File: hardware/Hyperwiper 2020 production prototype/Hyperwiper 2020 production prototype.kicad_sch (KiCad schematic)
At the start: 19 parts, among them K1 Main Power relay, K2 Wiper control relay, Q1 PN2222A, SW1 ON-OFF, U1 Teensy4.0, U3 L7805

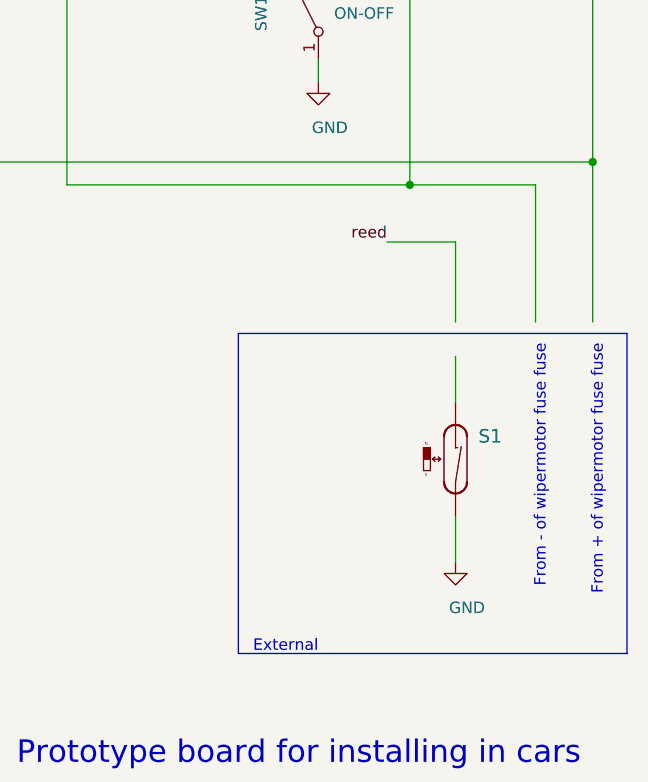
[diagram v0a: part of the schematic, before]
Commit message: Updated Schematic and board.
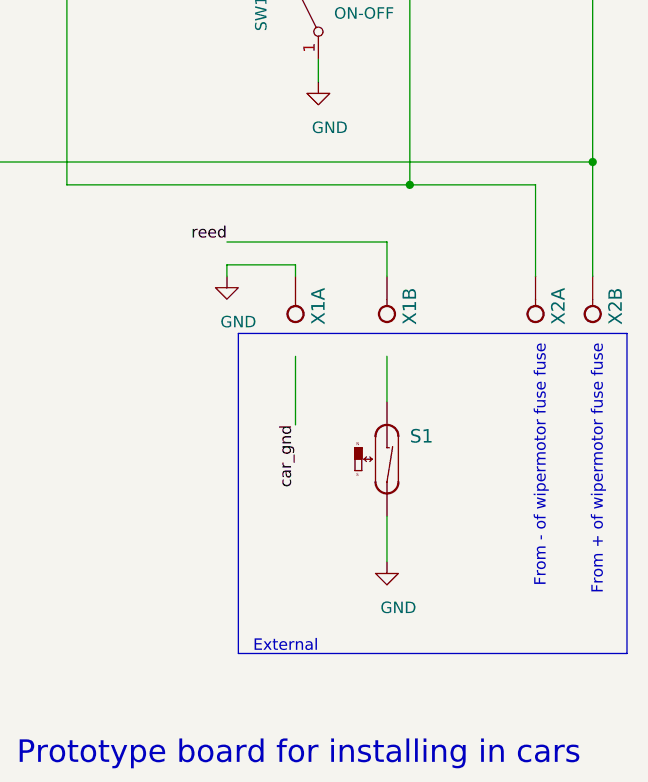
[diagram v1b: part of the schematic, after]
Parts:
- added X1, X2: W237-3E-bGeigieNanoKit_V1.1r5a-eagle-import, DWP 2020:W237-3E, symbol import_from_eagle-rescue:W237-3E-bGeigieNanoKit_V1.1r5a-eagle-import
- RV1: footprint Potentiometer_THT:Potentiometer_Alps_RK09K_Single_Horizontal -> Potentiometer_THT:Potentiometer_Piher_PT-10-V05_Vertical
- U3: footprint Package_TO_SOT_THT:TO-220-3_Vertical -> Package_TO_SOT_THT:TO-220-3_Horizontal_TabUp
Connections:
- net GND: now also X1.1 (KL)
- net reed: now also X1.2 (KL)
- net at K1.1, K2.3: now also X2.1 (KL)
- net at K1.4, K1.5, K2.1: now also X2.2 (KL)
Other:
- moved on the sheet: S1
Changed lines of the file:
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@@
+    (stroke (width 0) (type solid) (color 0 0 0 0))
+  )
+  (wire (pts (xy 234.95 114.3) (xy 252.73 114.3))
+    (stroke (width 0) (type solid) (color 0 0 0 0))
+  )
+  (wire (pts (xy 234.95 116.84) (xy 242.57 116.84))
+    (stroke (width 0) (type solid) (color 0 0 0 0))
+  )
+  (wire (pts (xy 234.95 118.11) (xy 234.95 116.84))
     (stroke (width 0) (type solid) (color 0 0 0 0))
   )
@@
     (stroke (width 0) (type solid) (color 0 0 0 0))
   )
+  (wire (pts (xy 242.57 116.84) (xy 242.57 118.11))
+    (stroke (width 0) (type solid) (color 0 0 0 0))
+  )
+  (wire (pts (xy 242.57 127) (xy 242.57 134.62))
+    (stroke (width 0) (type solid) (color 0 0 0 0))
+  )
   (wire (pts (xy 245.11 52.07) (xy 252.73 52.07))
     (stroke (width 0) (type solid) (color 0 0 0 0))
@@
     (stroke (width 0) (type solid) (color 0 0 0 0))
   )
-  (wire (pts (xy 252.73 114.3) (xy 260.35 114.3))
+  (wire (pts (xy 252.73 114.3) (xy 252.73 118.11))
+    (stroke (width 0) (type solid) (color 0 0 0 0))
+  )
+  (wire (pts (xy 252.73 127) (xy 252.73 132.08))
+    (stroke (width 0) (type solid) (color 0 0 0 0))
+  )
+  (wire (pts (xy 252.73 144.78) (xy 252.73 149.86))
     (stroke (width 0) (type solid) (color 0 0 0 0))
   )
@@
     (stroke (width 0) (type solid) (color 0 0 0 0))
   )
-  (wire (pts (xy 260.35 123.19) (xy 260.35 114.3))
-    (stroke (width 0) (type solid) (color 0 0 0 0))
-  )
-  (wire (pts (xy 260.35 127) (xy 260.35 132.08))
-    (stroke (width 0) (type solid) (color 0 0 0 0))
-  )
-  (wire (pts (xy 260.35 144.78) (xy 260.35 149.86))
-    (stroke (width 0) (type solid) (color 0 0 0 0))
-  )
-  (wire (pts (xy 269.24 107.95) (xy 269.24 123.19))
+  (wire (pts (xy 269.24 107.95) (xy 269.24 118.11))
     (stroke (width 0) (type solid) (color 0 0 0 0))
   )
@@
     (stroke (width 0) (type solid) (color 0 0 0 0))
   )
-  (wire (pts (xy 275.59 105.41) (xy 275.59 123.19))
+  (wire (pts (xy 275.59 105.41) (xy 275.59 118.11))
     (stroke (width 0) (type solid) (color 0 0 0 0))
   )
@@
     (effects (font (size 1.27 1.27)) (justify right bottom))
   )
+  (label "reed" (at 234.95 114.3 180)
+    (effects (font (size 1.27 1.27)) (justify right bottom))
+  )
+  (label "car_gnd" (at 242.57 134.62 270)
+    (effects (font (size 1.27 1.27)) (justify right bottom))
+  )
   (label "5V" (at 248.92 20.32 180)
     (effects (font (size 1.27 1.27)) (justify right bottom))
   )
-  (label "reed" (at 252.73 114.3 180)
-    (effects (font (size 1.27 1.27)) (justify right bottom))
-  )
   (symbol (lib_id "power:GND") (at 118.11 86.36 0) (unit 1)
     (in_bom yes) (on_board yes)
-    (property "Reference" "#PWR?" (id 0) (at 118.11 92.71 0)
+    (property "Reference" "#PWR0109" (id 0) (at 118.11 92.71 0)
       (effects (font (size 1.27 1.27)) hide)
     )
@@
     )
   )
+  (symbol (lib_id "power:GND") (at 234.95 118.11 0) (unit 1)
+    (in_bom yes) (on_board yes)
+    (property "Reference" "#PWR0110" (id 0) (at 234.95 124.46 0)
+      (effects (font (size 1.27 1.27)) hide)
+    )
+    (property "Value" "GND" (id 1) (at 236.22 123.19 0))
+    (property "Footprint" "" (id 2) (at 234.95 118.11 0)
+      (effects (font (size 1.27 1.27)) hide)
+    )
+    (property "Datasheet" "" (id 3) (at 234.95 118.11 0)
+      (effects (font (size 1.27 1.27)) hide)
+    )
+  )
   (symbol (lib_id "power:GND") (at 241.3 40.64 0) (unit 1)
     (in_bom yes) (on_board yes)
@@
     )
   )
-  (symbol (lib_id "power:GND") (at 260.35 149.86 0) (unit 1)
-    (in_bom yes) (on_board yes)
-    (property "Reference" "#PWR0104" (id 0) (at 260.35 156.21 0)
-      (effects (font (size 1.27 1.27)) hide)
-    )
-    (property "Value" "GND" (id 1) (at 261.62 154.94 0))
-    (property "Footprint" "" (id 2) (at 260.35 149.86 0)
-      (effects (font (size 1.27 1.27)) hide)
-    )
-    (property "Datasheet" "" (id 3) (at 260.35 149.86 0)
+  (symbol (lib_id "power:GND") (at 252.73 149.86 0) (unit 1)
+    (in_bom yes) (on_board yes)
+    (property "Reference" "#PWR0104" (id 0) (at 252.73 156.21 0)
+      (effects (font (size 1.27 1.27)) hide)
+    )
+    (property "Value" "GND" (id 1) (at 254 154.94 0))
+    (property "Footprint" "" (id 2) (at 252.73 149.86 0)
+      (effects (font (size 1.27 1.27)) hide)
+    )
+    (property "Datasheet" "" (id 3) (at 252.73 149.86 0)
+      (effects (font (size 1.27 1.27)) hide)
+    )
+  )
+  (symbol (lib_id "import_from_eagle-rescue:W237-3E-bGeigieNanoKit_V1.1r5a-eagle-import") (at 242.57 123.19 90) (unit 1)
+    (in_bom yes) (on_board yes)
+    (property "Reference" "X1" (id 0) (at 245.11 119.38 0)
+      (effects (font (size 1.4986 1.4986)) (justify right))
+    )
+    (property "Value" "W237-3E-bGeigieNanoKit_V1.1r5a-eagle-import" (id 1) (at 245.11 121.92 90)
+      (effects (font (size 1.499 1.499)) (justify right) hide)
+    )
+    (property "Footprint" "DWP 2020:W237-3E" (id 2) (at 242.57 123.19 0)
+      (effects (font (size 1.27 1.27)) hide)
+    )
+    (property "Datasheet" "" (id 3) (at 242.57 123.19 0)
+      (effects (font (size 1.27 1.27)) hide)
+    )
+  )
+  (symbol (lib_id "import_from_eagle-rescue:W237-3E-bGeigieNanoKit_V1.1r5a-eagle-import") (at 252.73 123.19 90) (unit 2)
+    (in_bom yes) (on_board yes)
+    (property "Reference" "X1" (id 0) (at 255.27 119.38 0)
+      (effects (font (size 1.4986 1.4986)) (justify right))
+    )
+    (property "Value" "W237-3E-bGeigieNanoKit_V1.1r5a-eagle-import" (id 1) (at 255.27 121.92 90)
+      (effects (font (size 1.499 1.499)) (justify right) hide)
+    )
+    (property "Footprint" "DWP 2020:W237-3E" (id 2) (at 252.73 123.19 0)
+      (effects (font (size 1.27 1.27)) hide)
+    )
+    (property "Datasheet" "" (id 3) (at 252.73 123.19 0)
+      (effects (font (size 1.27 1.27)) hide)
+    )
+  )
+  (symbol (lib_id "import_from_eagle-rescue:W237-3E-bGeigieNanoKit_V1.1r5a-eagle-import") (at 269.24 123.19 90) (unit 1)
+    (in_bom yes) (on_board yes)
+    (property "Reference" "X2" (id 0) (at 271.78 119.38 0)
+      (effects (font (size 1.4986 1.4986)) (justify right))
+    )
+    (property "Value" "W237-3E-bGeigieNanoKit_V1.1r5a-eagle-import" (id 1) (at 271.78 121.92 90)
+      (effects (font (size 1.499 1.499)) (justify right) hide)
+    )
+    (property "Footprint" "DWP 2020:W237-3E" (id 2) (at 269.24 123.19 0)
+      (effects (font (size 1.27 1.27)) hide)
+    )
+    (property "Datasheet" "" (id 3) (at 269.24 123.19 0)
+      (effects (font (size 1.27 1.27)) hide)
+    )
+  )
+  (symbol (lib_id "import_from_eagle-rescue:W237-3E-bGeigieNanoKit_V1.1r5a-eagle-import") (at 275.59 123.19 90) (unit 2)
+    (in_bom yes) (on_board yes)
+    (property "Reference" "X2" (id 0) (at 278.13 119.38 0)
+      (effects (font (size 1.4986 1.4986)) (justify right))
+    )
+    (property "Value" "W237-3E-bGeigieNanoKit_V1.1r5a-eagle-import" (id 1) (at 278.13 121.92 90)
+      (effects (font (size 1.499 1.499)) (justify right) hide)
+    )
+    (property "Footprint" "DWP 2020:W237-3E" (id 2) (at 275.59 123.19 0)
+      (effects (font (size 1.27 1.27)) hide)
+    )
+    (property "Datasheet" "" (id 3) (at 275.59 123.19 0)
       (effects (font (size 1.27 1.27)) hide)
     )
@@
       (effects (font (size 1.27 1.27)) (justify right))
     )
-    (property "Footprint" "Potentiometer_THT:Potentiometer_Alps_RK09K_Single_Horizontal" (id 2) (at 161.29 160.02 0)
+    (property "Footprint" "Potentiometer_THT:Potentiometer_Piher_PT-10-V05_Vertical" (id 2) (at 161.29 160.02 0)
       (effects (font (size 1.27 1.27)) hide)
     )
@@
     )
   )
-  (symbol (lib_id "import_from_eagle-rescue:REED-SWITCH-CT10-A2-bGeigieNanoKit_V1.1r5a-eagle-import") (at 260.35 139.7 0) (unit 1)
-    (in_bom yes) (on_board yes)
-    (property "Reference" "S1" (id 0) (at 262.89 135.89 0)
+  (symbol (lib_id "import_from_eagle-rescue:REED-SWITCH-CT10-A2-bGeigieNanoKit_V1.1r5a-eagle-import") (at 252.73 139.7 0) (unit 1)
+    (in_bom yes) (on_board yes)
+    (property "Reference" "S1" (id 0) (at 255.27 135.89 0)
       (effects (font (size 1.4986 1.4986)) (justify left))
     )
-    (property "Value" "REED-SWITCH-CT10-A2-bGeigieNanoKit_V1.1r5a-eagle-import" (id 1) (at 262.89 139.7 0)
+    (property "Value" "REED-SWITCH-CT10-A2-bGeigieNanoKit_V1.1r5a-eagle-import" (id 1) (at 255.27 139.7 0)
       (effects (font (size 1.499 1.499)) (justify left) hide)
     )
-    (property "Footprint" "" (id 2) (at 260.35 139.7 0)
-      (effects (font (size 1.27 1.27)) hide)
-    )
-    (property "Datasheet" "" (id 3) (at 260.35 139.7 0)
+    (property "Footprint" "" (id 2) (at 252.73 139.7 0)
+      (effects (font (size 1.27 1.27)) hide)
+    )
+    (property "Datasheet" "" (id 3) (at 252.73 139.7 0)
       (effects (font (size 1.27 1.27)) hide)
     )
@@
     (property "Reference" "U3" (id 0) (at 241.3 21.59 0))
     (property "Value" "L7805" (id 1) (at 241.3 24.13 0))
-    (property "Footprint" "Package_TO_SOT_THT:TO-220-3_Vertical" (id 2) (at 241.935 33.02 0)
+    (property "Footprint" "Package_TO_SOT_THT:TO-220-3_Horizontal_TabUp" (id 2) (at 241.935 33.02 0)
       (effects (font (size 1.27 1.27) italic) (justify left) hide)
     )
@@
     )
     (path "/9b49453a-7d8c-46f7-ac72-5b7ca2259e26"
-      (reference "#PWR?") (unit 1)
+      (reference "#PWR0109") (unit 1)
+    )
+    (path "/8e8791e7-f5c8-46ac-8494-bdb46b4d3074"
+      (reference "#PWR0110") (unit 1)
     )
     (path "/3e7c7f71-990b-4b23-8faa-21bc92ed5e62"
@@
       (reference "U3") (unit 1)
     )
-  )
+    (path "/a84228e8-43cd-4089-b680-2e81d592d20a"
+      (reference "X1") (unit 1)
+    )
+    (path "/20235294-3224-4d0b-9ea7-1bc2750028c9"
+      (reference "X1") (unit 2)
+    )
+    (path "/7b8a6e5c-ae62-44de-ab03-2dc22e81d347"
+      (reference "X2") (unit 1)
+    )
+    (path "/0c382f83-c9eb-437e-a290-b66c0c4bdbe8"
+      (reference "X2") (unit 2)
+    )
+  )

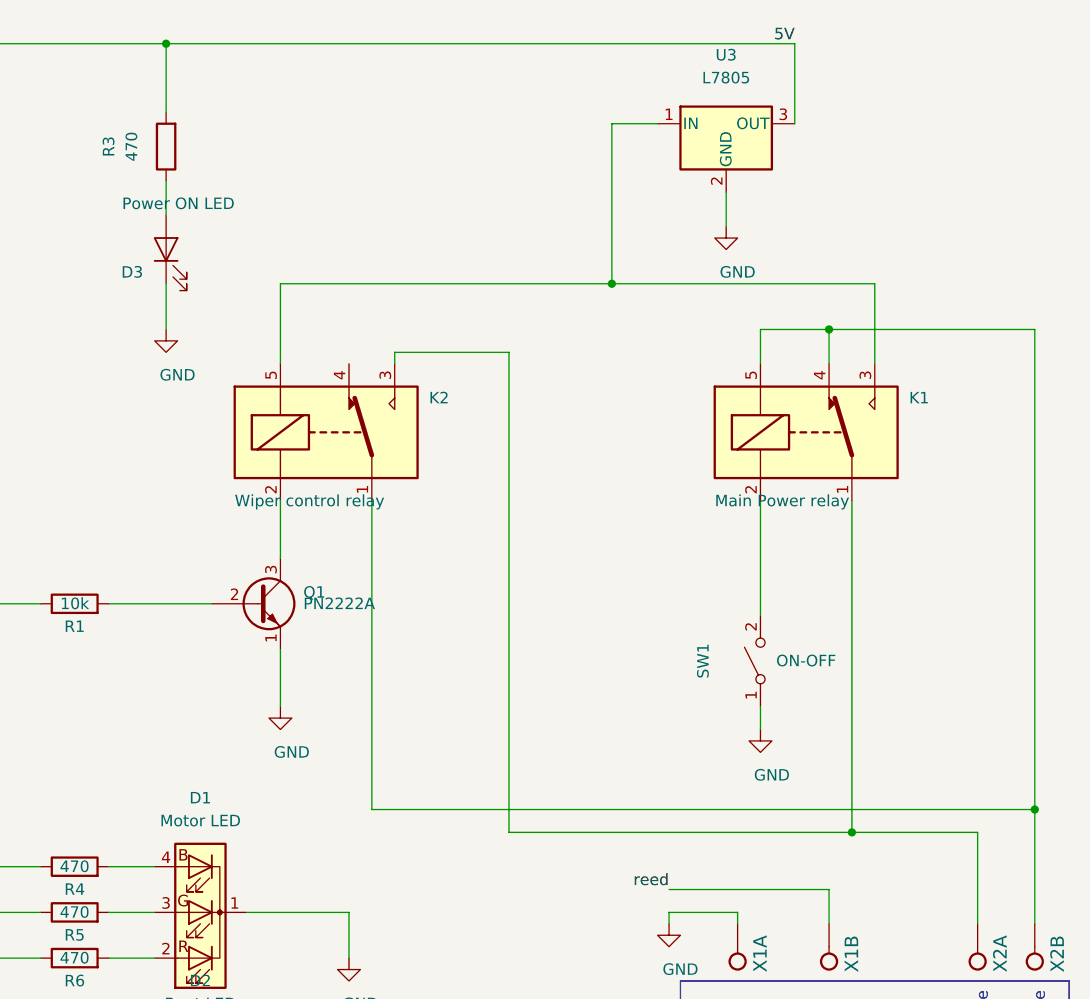
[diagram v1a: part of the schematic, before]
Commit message: updated kicad files with new traced board
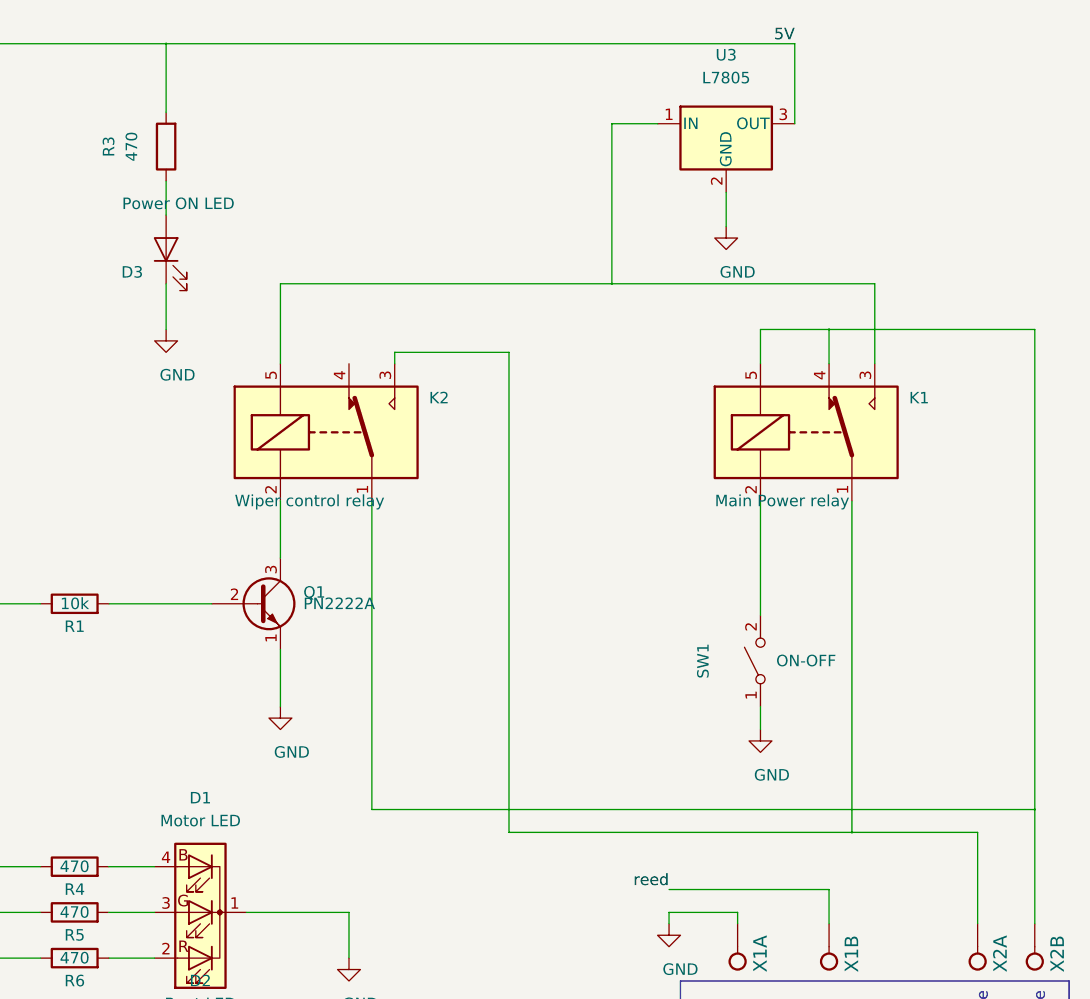
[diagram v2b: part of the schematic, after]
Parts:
- U3: footprint Package_TO_SOT_THT:TO-220-3_Horizontal_TabUp -> Package_TO_SOT_THT:TO-220-3_Vertical
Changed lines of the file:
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@@
-(kicad_sch (version 20200714) (host eeschema "5.99.0-unknown-a61ea1f~89~ubuntu20.04.1")
+(kicad_sch (version 20200714) (host eeschema "5.99.0-unknown-27d319b2d~89~ubuntu20.04.1")
   (page 1 1)
   (paper "A4")
@@
     (date "2020-07-25")
   )
-  (junction (at 179.07 20.32) (diameter 0) (color 0 0 0 0))
-  (junction (at 228.6 46.99) (diameter 0) (color 0 0 0 0))
-  (junction (at 252.73 52.07) (diameter 0) (color 0 0 0 0))
-  (junction (at 255.27 107.95) (diameter 0) (color 0 0 0 0))
-  (junction (at 275.59 105.41) (diameter 0) (color 0 0 0 0))
+  (junction (at 179.07 20.32) (diameter 0.2591) (color 0 0 0 0))
+  (junction (at 228.6 46.99) (diameter 0.2591) (color 0 0 0 0))
+  (junction (at 252.73 52.07) (diameter 0.2591) (color 0 0 0 0))
+  (junction (at 255.27 107.95) (diameter 0.2591) (color 0 0 0 0))
+  (junction (at 275.59 105.41) (diameter 0.2591) (color 0 0 0 0))
   (wire (pts (xy 107.95 83.82) (xy 140.97 83.82))
     (stroke (width 0) (type solid) (color 0 0 0 0))
@@
     (property "Reference" "U3" (id 0) (at 241.3 21.59 0))
     (property "Value" "L7805" (id 1) (at 241.3 24.13 0))
-    (property "Footprint" "Package_TO_SOT_THT:TO-220-3_Horizontal_TabUp" (id 2) (at 241.935 33.02 0)
+    (property "Footprint" "Package_TO_SOT_THT:TO-220-3_Vertical" (id 2) (at 241.935 33.02 0)
       (effects (font (size 1.27 1.27) italic) (justify left) hide)
     )
